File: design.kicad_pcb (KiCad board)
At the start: 2 copper layers, 35.1 x 15 mm, 20 parts, among them J1 USB_C_Receptacle, J2 Conn_01x05, Q1 2N7002K, Q2 2N7002K, Q3 2N7002K, U1 ATtiny814-SS

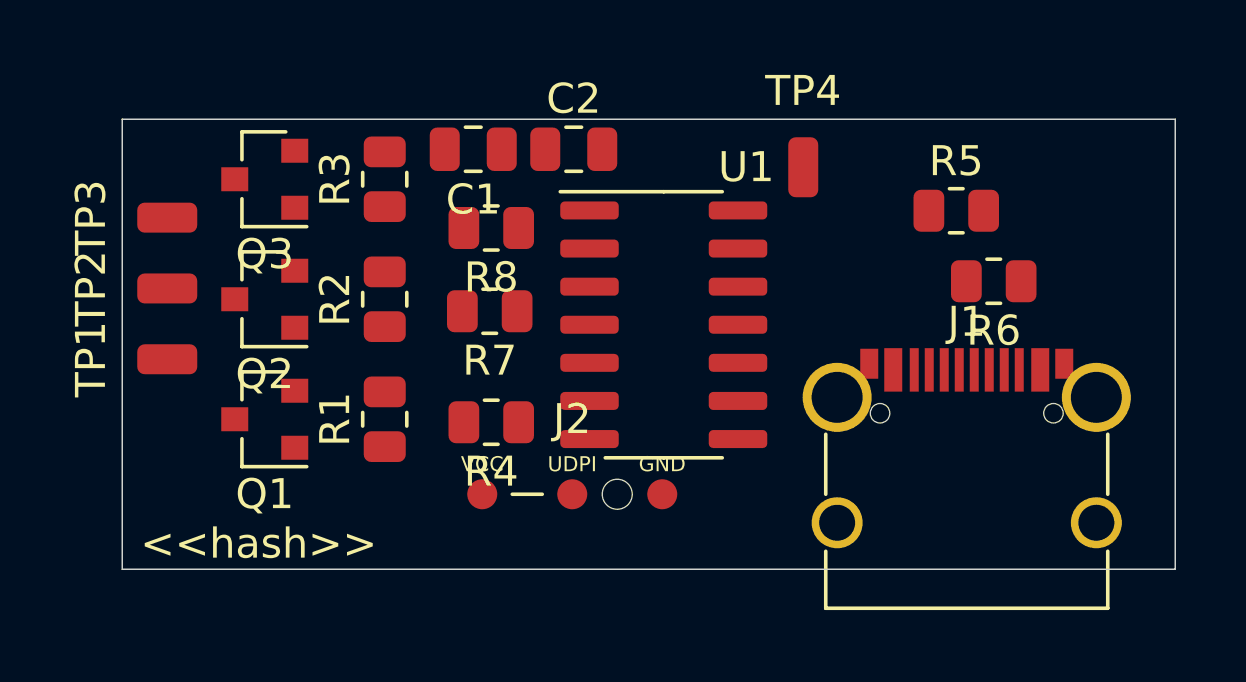
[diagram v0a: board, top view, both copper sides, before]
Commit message: PCB: arrange
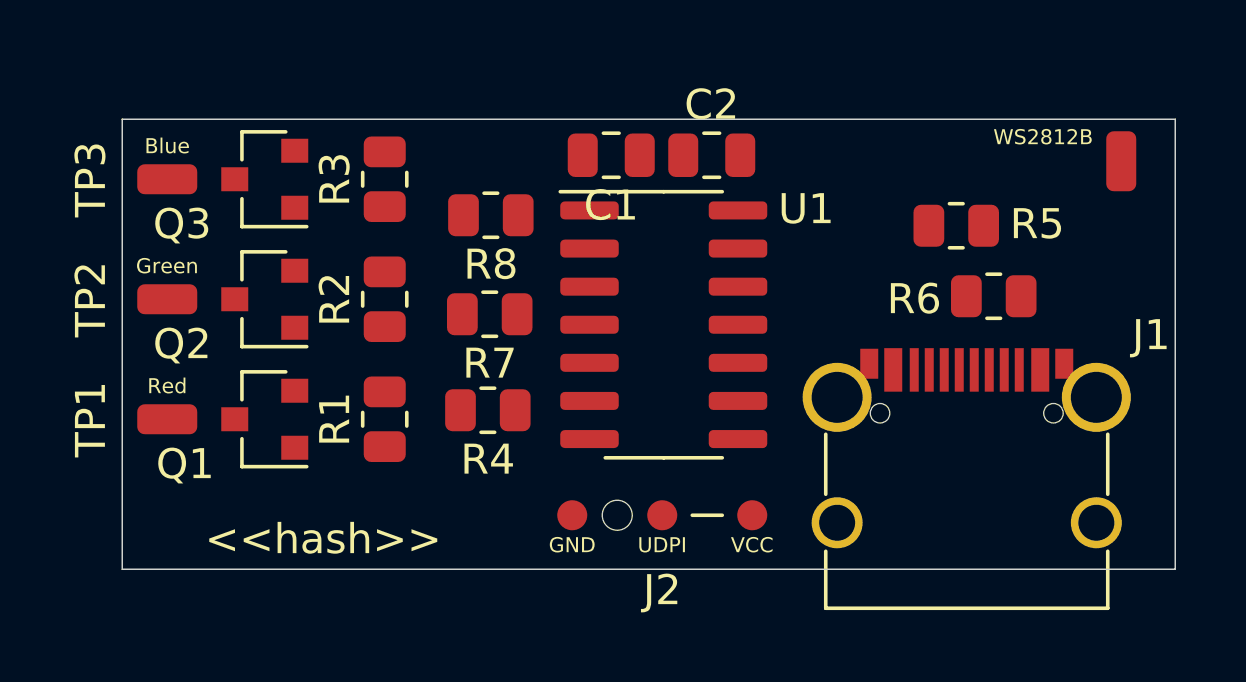
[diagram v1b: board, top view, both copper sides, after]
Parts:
- moved TP4 10.6 mm to (169.8, 81.4)
- moved C1 4.60 mm to (152.8, 81.2)
- moved C2 4.60 mm to (156.2, 81.2)
- moved J2 3.08 mm to (154.5, 93.2), turned to 180 degrees
- moved TP1 2.00 mm to (138.0, 90.0)
- moved TP3 1.28 mm to (138.0, 82.0)
- moved R5 0.50 mm to (164.3, 83.5)
- moved R6 0.50 mm to (165.6, 85.9)
- moved R8 0.43 mm to (148.8, 83.2)
- moved R4 0.42 mm to (148.7, 89.7)
- moved TP2 0.36 mm to (138.0, 86.0)
- moved R7 0.10 mm to (148.8, 86.5)
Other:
- board text added: "Blue"
- board text added: "Green"
- board text added: "Red"
- board text added: "WS2812B"
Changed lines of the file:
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@@
   (general
     (thickness 1.6)
-    (drawings 6)
+    (drawings 10)
     (tracks 0)
     (zones 0)
@@
     (47 F.CrtYd user)
     (48 B.Fab user)
-    (49 F.Fab user)
+    (49 F.Fab user hide)
   )
   (setup
@@
   )
   (module Resistor_SMD:R_0805_2012Metric (layer F.Cu)
-    (at 148.8 83.625 180)
+    (at 148.7875 83.2 180)
     (descr "Resistor SMD 0805 (2012 Metric), square (rectangular) end terminal, IPC_7351 nominal, (Body size source: IPC-SM-782 page 72, https://www.pcb-3d.com/wordpress/wp-content/uploads/ipc-sm-782a_amendment_1_and_2.pdf), generated with kicad-footprint-generator")
     (tags resistor)
@@
   )
   (module Resistor_SMD:R_0805_2012Metric (layer F.Cu)
-    (at 148.75 86.4 180)
+    (at 148.75 86.5 180)
     (descr "Resistor SMD 0805 (2012 Metric), square (rectangular) end terminal, IPC_7351 nominal, (Body size source: IPC-SM-782 page 72, https://www.pcb-3d.com/wordpress/wp-content/uploads/ipc-sm-782a_amendment_1_and_2.pdf), generated with kicad-footprint-generator")
     (tags resistor)
@@
   )
   (module Resistor_SMD:R_0805_2012Metric (layer F.Cu)
-    (at 165.55 85.4 180)
+    (at 165.55 85.9 180)
     (descr "Resistor SMD 0805 (2012 Metric), square (rectangular) end terminal, IPC_7351 nominal, (Body size source: IPC-SM-782 page 72, https://www.pcb-3d.com/wordpress/wp-content/uploads/ipc-sm-782a_amendment_1_and_2.pdf), generated with kicad-footprint-generator")
     (tags resistor)
     (attr smd)
-    (fp_text reference R6 (at 0 -1.65) (layer F.SilkS)
+    (fp_text reference R6 (at 2.65 -0.1) (layer F.SilkS)
       (effects (font (size 1 1) (thickness 0.15)))
     )
@@
   )
   (module Resistor_SMD:R_0805_2012Metric (layer F.Cu)
-    (at 164.3 83.05)
+    (at 164.3 83.55)
     (descr "Resistor SMD 0805 (2012 Metric), square (rectangular) end terminal, IPC_7351 nominal, (Body size source: IPC-SM-782 page 72, https://www.pcb-3d.com/wordpress/wp-content/uploads/ipc-sm-782a_amendment_1_and_2.pdf), generated with kicad-footprint-generator")
     (tags resistor)
     (attr smd)
-    (fp_text reference R5 (at 0 -1.65) (layer F.SilkS)
+    (fp_text reference R5 (at 2.7 -0.05) (layer F.SilkS)
       (effects (font (size 1 1) (thickness 0.15)))
     )
@@
   )
   (module Resistor_SMD:R_0805_2012Metric (layer F.Cu)
-    (at 148.8 90.1 180)
+    (at 148.6875 89.7 180)
     (descr "Resistor SMD 0805 (2012 Metric), square (rectangular) end terminal, IPC_7351 nominal, (Body size source: IPC-SM-782 page 72, https://www.pcb-3d.com/wordpress/wp-content/uploads/ipc-sm-782a_amendment_1_and_2.pdf), generated with kicad-footprint-generator")
     (tags resistor)
@@
   )
   (module E32-xxxT20D:UDPI_interface_small (layer F.Cu)
-    (at 151.5 92.5)
+    (at 154.5 93.2 180)
     (fp_text reference J2 (at 0 -2.5) (layer F.SilkS)
       (effects (font (size 1 1) (thickness 0.15)))
@@
     )
     (fp_line (start -2 0) (end -1 0) (layer F.SilkS) (width 0.12))
-    (pad "" np_thru_hole circle (at 1.5 0) (size 1 1) (drill 1) (layers *.Cu *.Mask))
-    (pad 3 smd circle (at 3 0) (size 1 1) (layers F.Cu F.Paste F.Mask)
-      (net 15 GND))
-    (pad 2 smd circle (at -3 0) (size 1 1) (layers F.Cu F.Paste F.Mask)
+    (pad "" np_thru_hole circle (at 1.5 0 180) (size 1 1) (drill 1) (layers *.Cu *.Mask))
+    (pad 3 smd circle (at 3 0 180) (size 1 1) (layers F.Cu F.Paste F.Mask)
+      (net 15 GND))
+    (pad 2 smd circle (at -3 0 180) (size 1 1) (layers F.Cu F.Paste F.Mask)
       (net 22 VCC))
-    (pad 1 smd circle (at 0 0) (size 1 1) (layers F.Cu F.Paste F.Mask)
+    (pad 1 smd circle (at 0 0 180) (size 1 1) (layers F.Cu F.Paste F.Mask)
       (net 25 UDPI))
   )
@@
     (tags "usb usb-c 2.0 pd")
     (attr smd)
-    (fp_text reference J1 (at 0 -5.645) (layer F.SilkS)
+    (fp_text reference J1 (at 6.15 -5.2) (layer F.SilkS)
       (effects (font (size 1 1) (thickness 0.15)))
     )
@@
     (tags "SOIC SO")
     (attr smd)
-    (fp_text reference U1 (at 2.75 -5.25) (layer F.SilkS)
+    (fp_text reference U1 (at 4.75 -3.85) (layer F.SilkS)
       (effects (font (size 1 1) (thickness 0.15)))
     )
@@
   )
   (module Connector_Wire:SolderWirePad_1x01_SMD_1x2mm (layer F.Cu)
-    (at 159.2 81.6)
+    (at 169.8 81.4)
     (descr "Wire Pad, Square, SMD Pad,  5mm x 10mm,")
     (tags "MesurementPoint Square SMDPad 5mmx10mm ")
     (attr virtual)
-    (fp_text reference TP4 (at 0 -2.54) (layer F.SilkS)
+    (fp_text reference TP4 (at 0 -2.54) (layer F.SilkS) hide
       (effects (font (size 1 1) (thickness 0.15)))
     )
@@
   )
   (module Connector_Wire:SolderWirePad_1x01_SMD_1x2mm (layer F.Cu)
-    (at 138 83.28 90)
+    (at 138 82 90)
     (descr "Wire Pad, Square, SMD Pad,  5mm x 10mm,")
     (tags "MesurementPoint Square SMDPad 5mmx10mm ")
@@
   )
   (module Connector_Wire:SolderWirePad_1x01_SMD_1x2mm (layer F.Cu)
-    (at 138 85.64 90)
+    (at 138 86 90)
     (descr "Wire Pad, Square, SMD Pad,  5mm x 10mm,")
     (tags "MesurementPoint Square SMDPad 5mmx10mm ")
@@
   )
   (module Connector_Wire:SolderWirePad_1x01_SMD_1x2mm (layer F.Cu)
-    (at 138 88 90)
+    (at 138 90 90)
     (descr "Wire Pad, Square, SMD Pad,  5mm x 10mm,")
     (tags "MesurementPoint Square SMDPad 5mmx10mm ")
@@
     (tags SOT-23)
     (attr smd)
-    (fp_text reference Q3 (at 0 -2.5) (layer F.SilkS)
+    (fp_text reference Q3 (at 2.75 -1.5) (layer F.SilkS)
       (effects (font (size 1 1) (thickness 0.15)))
     )
@@
     (tags SOT-23)
     (attr smd)
-    (fp_text reference Q2 (at 0 -2.5) (layer F.SilkS)
+    (fp_text reference Q2 (at 2.75 -1.5) (layer F.SilkS)
       (effects (font (size 1 1) (thickness 0.15)))
     )
@@
     (tags SOT-23)
     (attr smd)
-    (fp_text reference Q1 (at 0 -2.5) (layer F.SilkS)
+    (fp_text reference Q1 (at 2.65 -1.5) (layer F.SilkS)
       (effects (font (size 1 1) (thickness 0.15)))
     )
@@
   )
   (module Capacitor_SMD:C_0805_2012Metric (layer F.Cu)
-    (at 151.55 81)
+    (at 156.15 81.2)
     (descr "Capacitor SMD 0805 (2012 Metric), square (rectangular) end terminal, IPC_7351 nominal, (Body size source: IPC-SM-782 page 76, https://www.pcb-3d.com/wordpress/wp-content/uploads/ipc-sm-782a_amendment_1_and_2.pdf, https://docs.google.com/spreadsheets/d/1BsfQQcO9C6DZCsRaXUlFlo91Tg2WpOkGARC1WS5S8t0/edit?usp=sharing), generated with kicad-footprint-generator")
     (tags capacitor)
@@
   )
   (module Capacitor_SMD:C_0805_2012Metric (layer F.Cu)
-    (at 148.2 81 180)
+    (at 152.8 81.2 180)
     (descr "Capacitor SMD 0805 (2012 Metric), square (rectangular) end terminal, IPC_7351 nominal, (Body size source: IPC-SM-782 page 76, https://www.pcb-3d.com/wordpress/wp-content/uploads/ipc-sm-782a_amendment_1_and_2.pdf, https://docs.google.com/spreadsheets/d/1BsfQQcO9C6DZCsRaXUlFlo91Tg2WpOkGARC1WS5S8t0/edit?usp=sharing), generated with kicad-footprint-generator")
     (tags capacitor)
@@
     )
   )
+  (gr_text WS2812B (at 167.2 80.6) (layer F.SilkS)
+    (effects (font (size 0.5 0.5) (thickness 0.1)))
+  )
+  (gr_text Red (at 138 88.9) (layer F.SilkS)
+    (effects (font (size 0.5 0.5) (thickness 0.1)))
+  )
+  (gr_text Green (at 138 84.9) (layer F.SilkS)
+    (effects (font (size 0.5 0.5) (thickness 0.1)))
+  )
+  (gr_text Blue (at 138 80.9) (layer F.SilkS)
+    (effects (font (size 0.5 0.5) (thickness 0.1)))
+  )
   (dimension 15 (width 0.15) (layer Dwgs.User)
     (gr_text "15.000 mm" (at 131.45 87.5 270) (layer Dwgs.User)
@@
     (arrow2b (pts (xy 132.75 80) (xy 133.336421 81.126504)))
   )
-  (gr_text <<hash>> (at 141.05 94.15) (layer F.SilkS)
+  (gr_text <<hash>> (at 143.2 94) (layer F.SilkS)
     (effects (font (size 1 1) (thickness 0.15)))
   )
